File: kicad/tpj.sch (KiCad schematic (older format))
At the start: 9 parts, among them P1 CONN_01X03, P2 USB_A, U1 LD1117S33TR, U2 ESP-12E

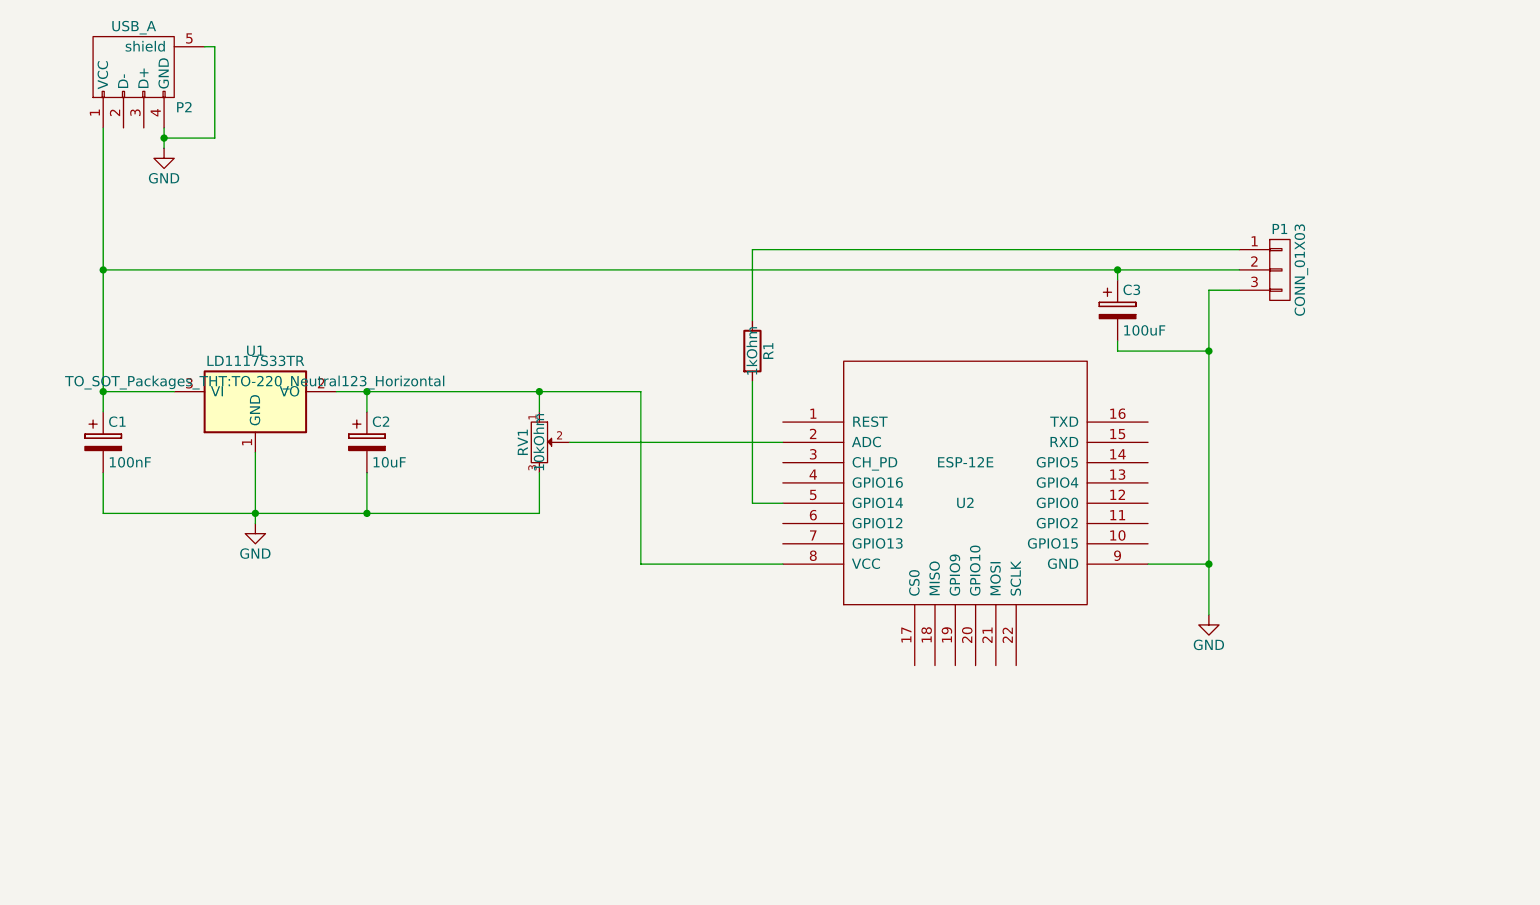
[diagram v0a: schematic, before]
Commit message: added schematic
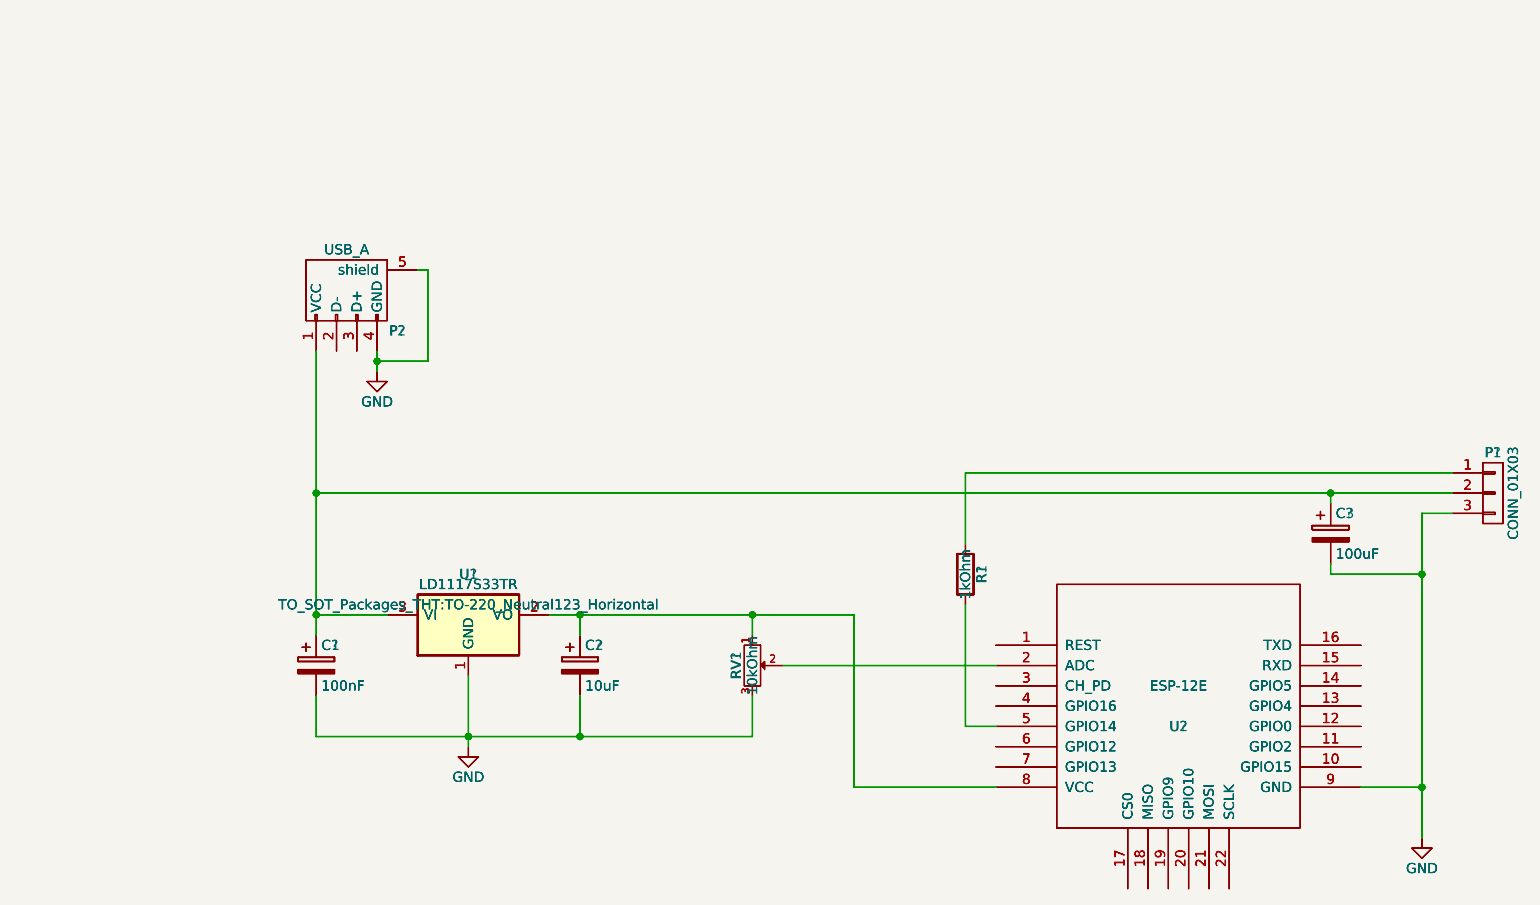
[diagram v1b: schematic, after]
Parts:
- added C?: 100uF, Capacitors_ThroughHole:C_Axial_D5_L11_P18, symbol CP
- added C?: 100nF, Capacitors_ThroughHole:C_Axial_D5_L11_P18, symbol CP
- added C?: 10uF, Capacitors_ThroughHole:C_Axial_D5_L11_P18, symbol CP
- added P?: CONN_01X03, Pin_Headers:Pin_Header_Angled_1x03, symbol CONN_01X03
- added P?: USB_A, Connect:USB_Micro-B, symbol USB_A
- added R?: 1kOhm, Resistors_ThroughHole:Resistor_Horizontal_RM7mm, symbol R
- added RV?: 10kOhm, Potentiometers:Potentiometer_WirePads_largePads, symbol POT
- added U?: ESP-12E, ESP8266:ESP-12E, symbol ESP-12E
- added U?: LD1117S33TR, TO_SOT_Packages_THT:TO-220_Neutral123_Horizontal, symbol LD1117S33TR
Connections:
- net GND: now also C?.2, C?.2, C?.2, P?.3 (P3), P?.4 (GND), P?.5 (shield), RV?.3, U?.1 (GND), U?.9 (GND)
- net at U2.1 (REST): now also U?.1 (REST)
- net at U2.10 (GPIO15): now also U?.10 (GPIO15)
- net at U2.11 (GPIO2): now also U?.11 (GPIO2)
- net at U2.12 (GPIO0): now also U?.12 (GPIO0)
- net at U2.13 (GPIO4): now also U?.13 (GPIO4)
- net at U2.14 (GPIO5): now also U?.14 (GPIO5)
- net at U2.15 (RXD): now also U?.15 (RXD)
- net at U2.16 (TXD): now also U?.16 (TXD)
- net at U2.17 (CS0): now also U?.17 (CS0)
- net at U2.18 (MISO): now also U?.18 (MISO)
- net at U2.19 (GPIO9): now also U?.19 (GPIO9)
- net at RV1.2, U2.2 (ADC): now also RV?.2, U?.2 (ADC)
- net at U2.20 (GPIO10): now also U?.20 (GPIO10)
- net at U2.21 (MOSI): now also U?.21 (MOSI)
- net at U2.22 (SCLK): now also U?.22 (SCLK)
- net at U2.3 (CH_PD): now also U?.3 (CH_PD)
- net at U2.4 (GPIO16): now also U?.4 (GPIO16)
- net at R1.2, U2.5 (GPIO14): now also R?.2, U?.5 (GPIO14)
- net at U2.6 (GPIO12): now also U?.6 (GPIO12)
- net at U2.7 (GPIO13): now also U?.7 (GPIO13)
- net at C2.1, RV1.1, U1.2 (VO)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: now also C?.1, RV?.1, U?.2 (VO), U?.8 (VCC)
- net at C1.1, C3.1, P1.2 (P2)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: now also C?.1, C?.1, P?.1 (VCC), P?.2 (P2), U?.3 (VI)
- net at P1.1 (P1), R1.1: now also P?.1 (P1), R?.1
- net at P2.2 (D-): now also P?.2 (D-)
- net at P2.3 (D+): now also P?.3 (D+)
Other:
- moved on the sheet: C1, C2, C3, P1, P2, R1, RV1, U1, U2
